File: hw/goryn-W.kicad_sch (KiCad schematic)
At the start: 4 parts, among them J1 Conn_01x34

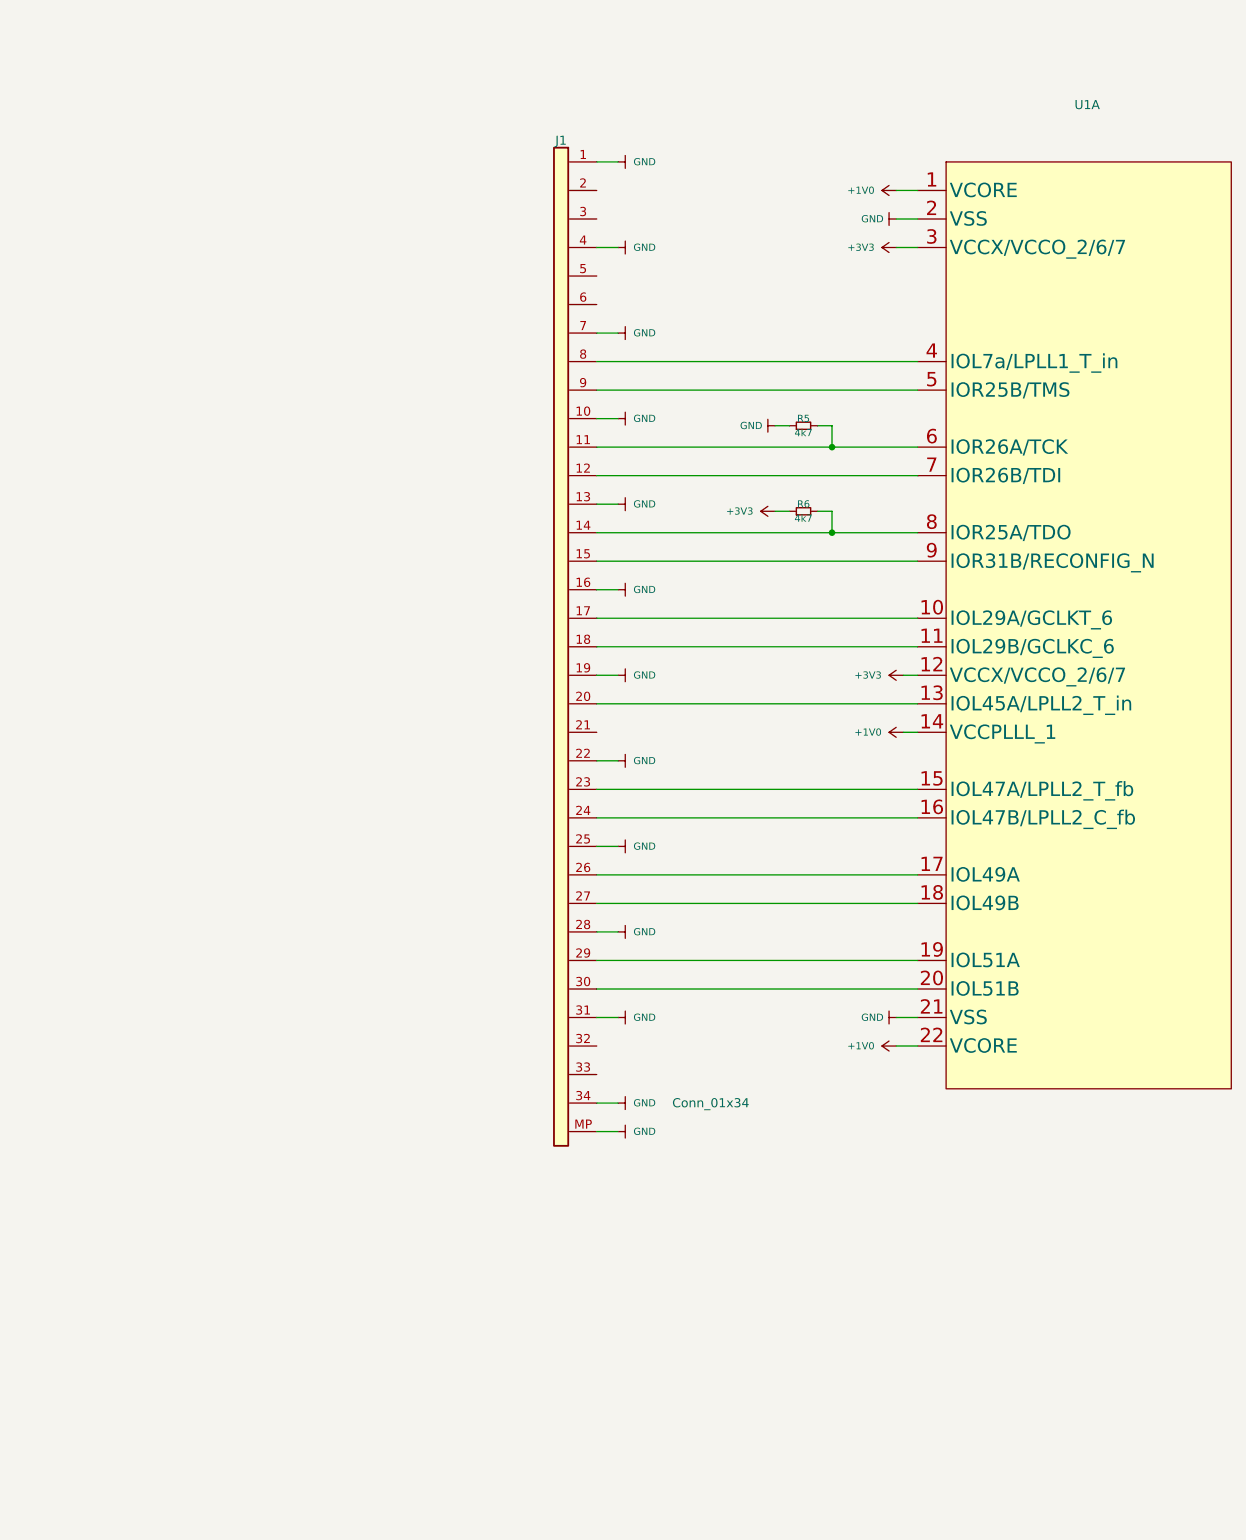
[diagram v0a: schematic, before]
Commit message: added DC-DC
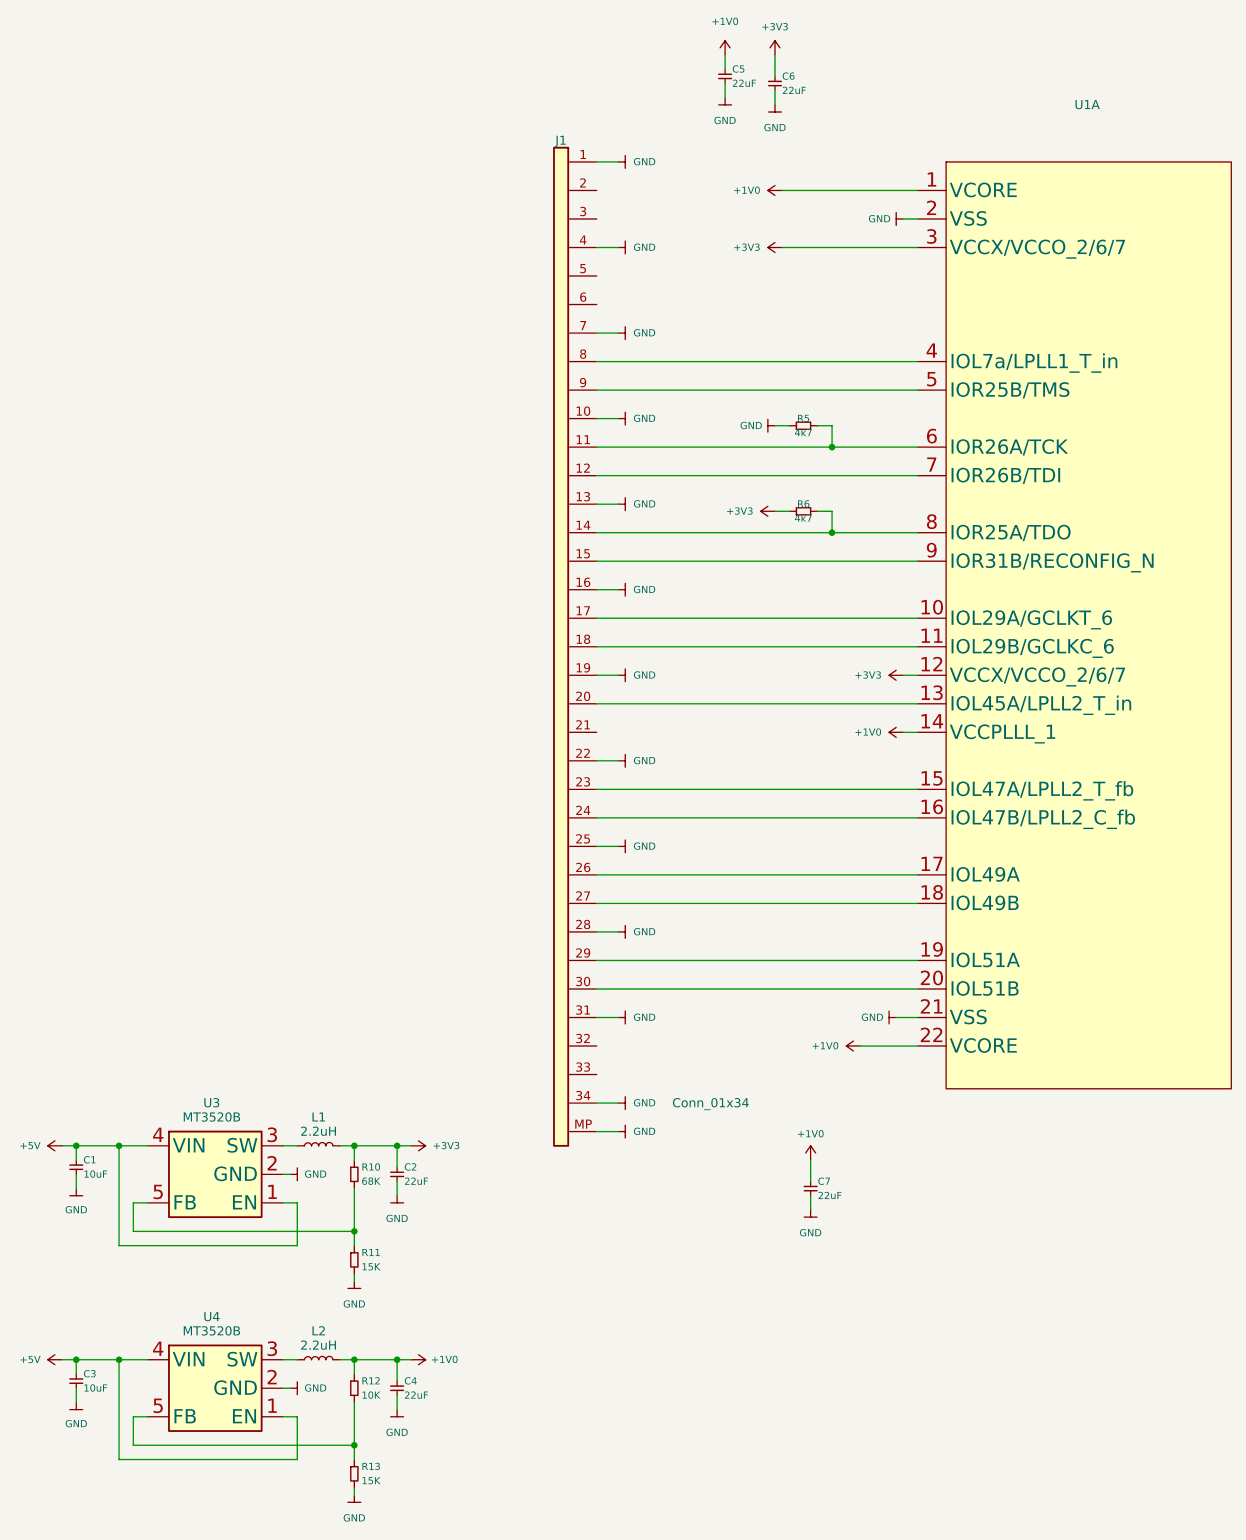
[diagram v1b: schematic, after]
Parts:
- added C1, C3: 10uF, AI6YP:C_0603_1608Metric, symbol AI6YP:C
- added C2, C4, C5, C6, C7: 22uF, AI6YP:C_0603_1608Metric, symbol AI6YP:C
- added L1, L2: 2.2uH, AI6YP:L_0805_2012Metric_Pad1.05x1.20mm_HandSolder, symbol AI6YP:L
- added R10: 68K, AI6YP:R_0603_1608Metric, symbol AI6YP:R
- added R11, R13: 15K, AI6YP:R_0603_1608Metric, symbol AI6YP:R
- added R12: 10K, AI6YP:R_0603_1608Metric, symbol AI6YP:R
- added U3, U4: MT3520B, AI6YP:SOT-23-5, symbol AI6YP:MT3520B
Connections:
- net +1V0: now also C4.1, C5.1, C7.1, L2.2, R12.1
- net +3V3: now also C2.1, C6.1, L1.2, R10.1
- net GND: now also C1.2, C2.2, C3.2, C4.2, C5.2, C6.2, C7.2, R11.2, R13.2, U3.2 (GND), U4.2 (GND)
- new net: L2.1, U4.3 (SW)
- new net: R12.2, R13.1, U4.5 (FB)
- new net: R10.2, R11.1, U3.5 (FB)
- new net: L1.1, U3.3 (SW)
- new net +5V: C1.1, C3.1, U3.1 (EN), U3.4 (VIN), U4.1 (EN), U4.4 (VIN)
